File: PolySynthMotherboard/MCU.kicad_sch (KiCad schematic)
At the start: 46 parts, among them J201 SWD Header, J202 USB_C, J203 MIDI_In, J204 MIDI_Thru, J207 MIDI_Out, J401 Micro_SD_Card_Det2, SW201 RST, SW202 BOOT, U201 STM32F411RETx, U202 74HC595, U203 74HC595, U204 6N138, U205 74HC04, Y201 16MHz, Y202 32.768kHZ

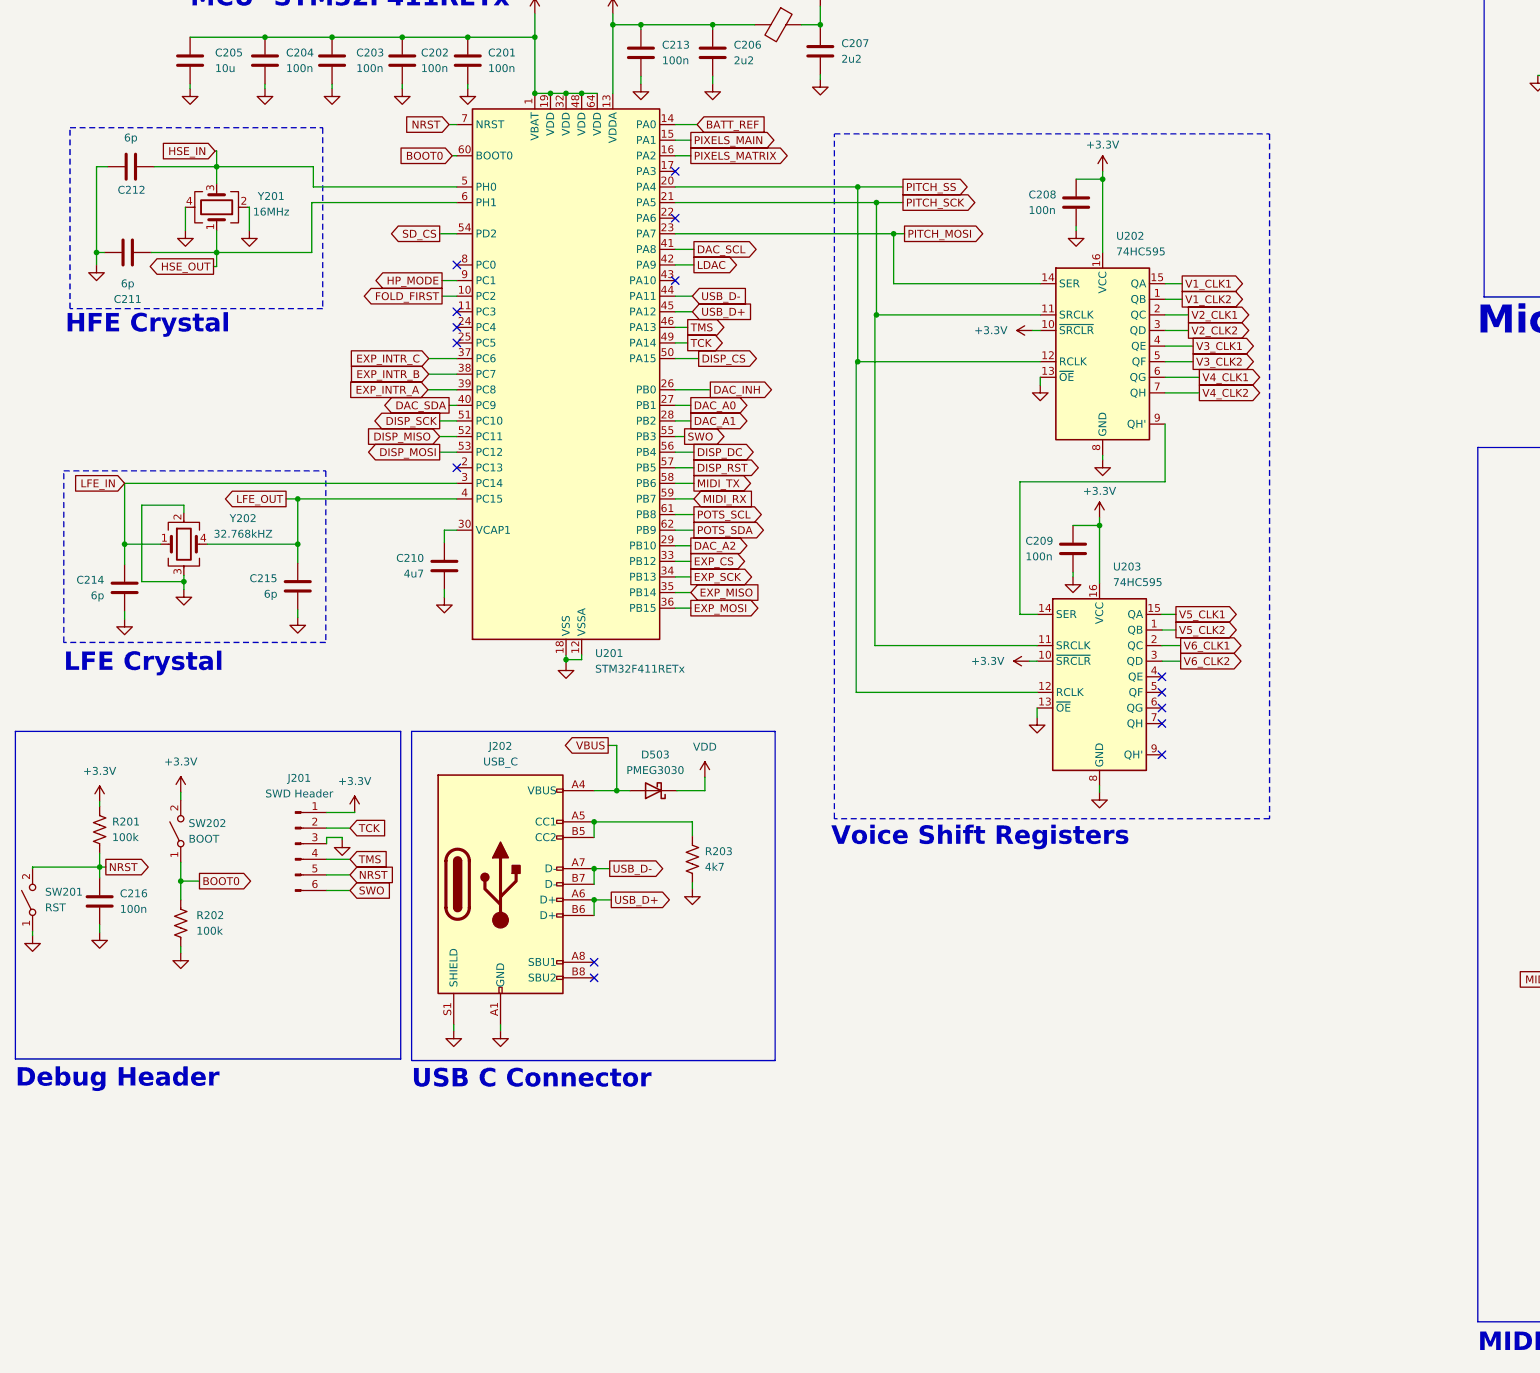
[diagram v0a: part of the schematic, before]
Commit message: added terminations
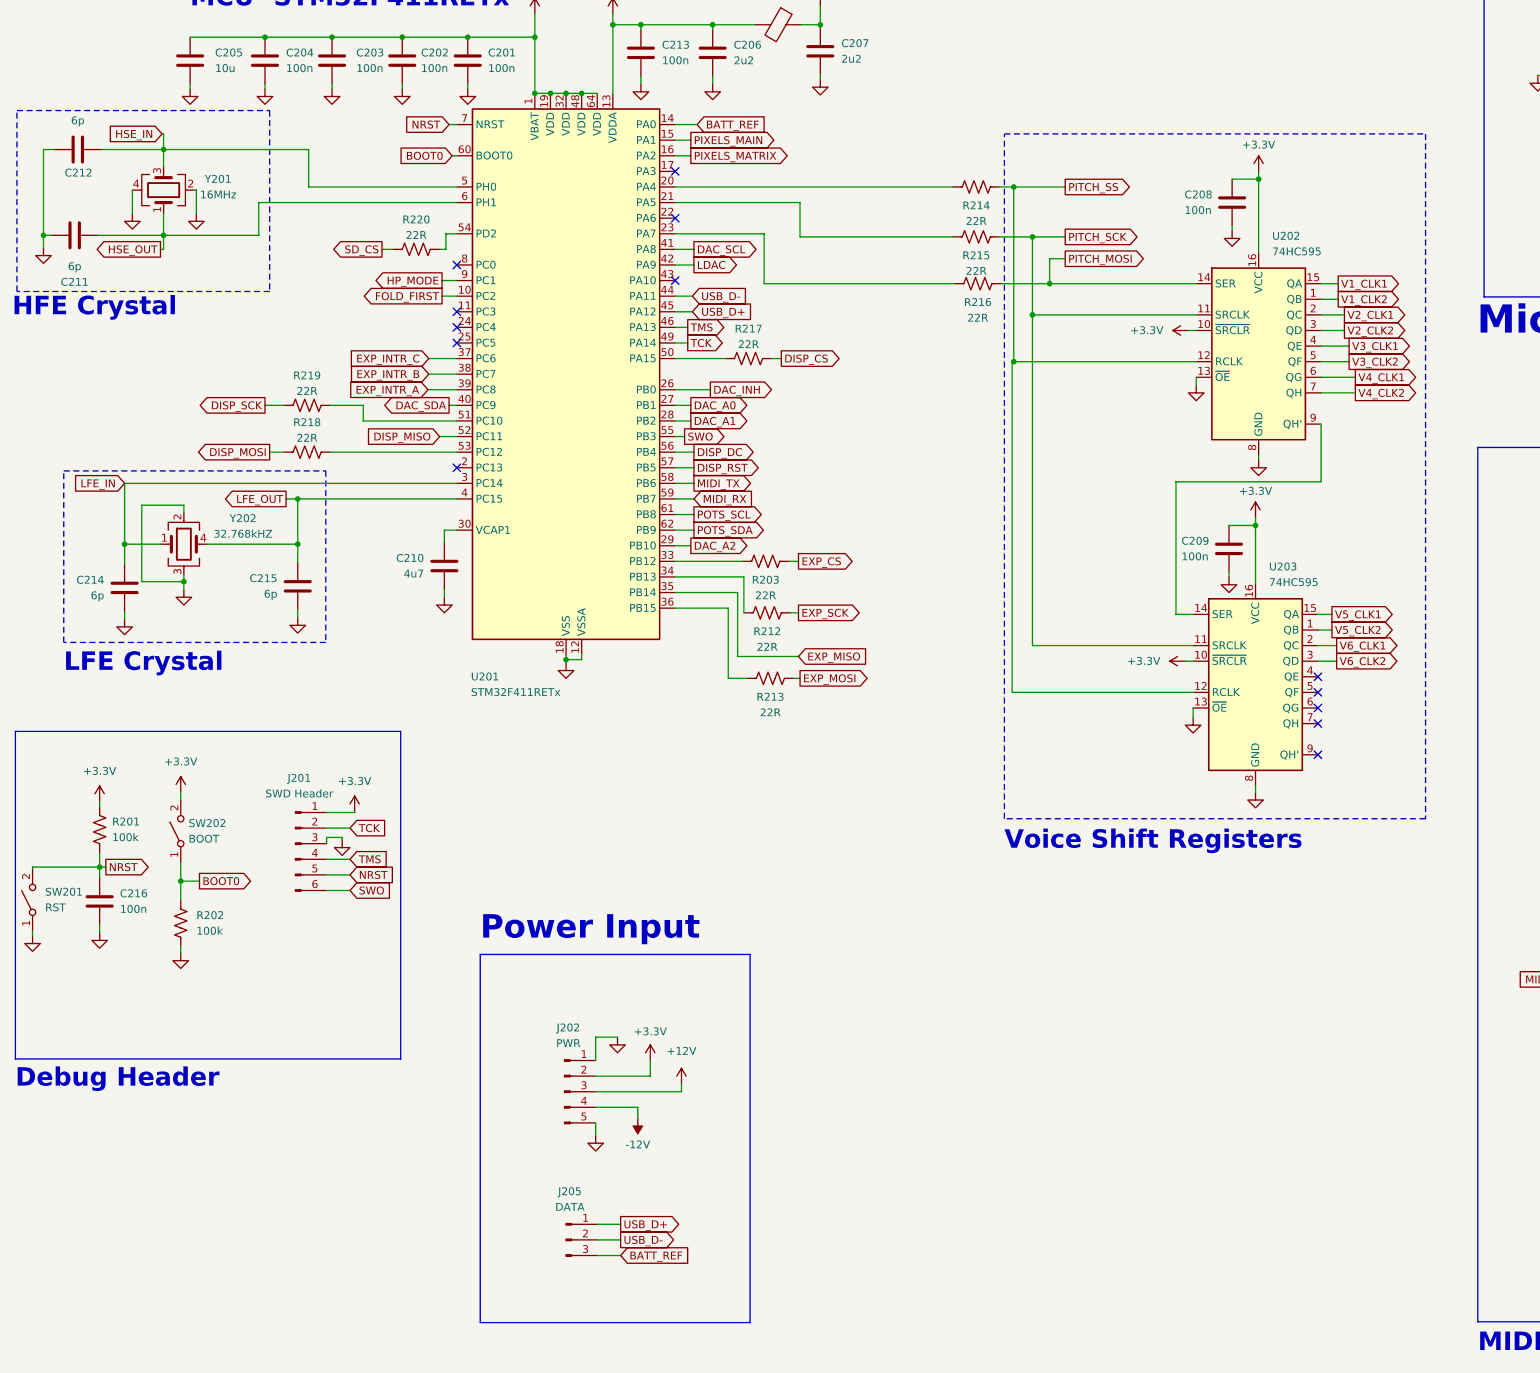
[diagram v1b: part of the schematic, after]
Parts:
- removed D503: PMEG3030, Diode_SMD:D_SOD-123, symbol Device:D_Schottky
- removed J202: USB_C, Connector_USB:USB_C_Receptacle_JAE_DX07S016JA1R1500, symbol Connector:USB_C_Receptacle_USB2.0
- added J202: PWR, Connector_PinHeader_2.54mm:PinHeader_1x05_P2.54mm_Vertical, symbol Connector:Conn_01x05_Pin
- added J205: DATA, Connector_PinHeader_2.54mm:PinHeader_1x03_P2.54mm_Vertical, symbol Connector:Conn_01x03_Pin
- added R212, R213, R214, R215, R216, R217, R218, R219, R220: 22R, Resistor_SMD:R_0805_2012Metric, symbol Device:R_US
- R203: value 4k7 -> 22R
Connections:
- net +3.3V: now also J202.2 (Pin_2)
- net BATT_REF: now also J205.3 (Pin_3)
- net DISP_CS: now also R217.2; no longer U201.50 (PA15)
- net DISP_MOSI: now also R218.1; no longer U201.53 (PC12)
- net DISP_SCK: now also R219.1; no longer U201.51 (PC10)
- net EXP_CS: now also R203.2; no longer U201.33 (PB12)
- net EXP_MOSI: now also R213.2; no longer U201.36 (PB15)
- net EXP_SCK: now also R212.2; no longer U201.34 (PB13)
- net GND: now also J202.1 (Pin_1), J202.5 (Pin_5); no longer R203.2
- net PITCH_MOSI: now also R216.2; no longer U201.23 (PA7)
- net PITCH_SCK: now also R215.2; no longer U201.21 (PA5)
- net PITCH_SS: now also R214.2; no longer U201.20 (PA4)
- net SD_CS: now also R220.1; no longer U201.54 (PD2)
- net USB_D+: now also J205.1 (Pin_1)
- net USB_D-: now also J205.2 (Pin_2)
- net at R203.1: now also U201.33 (PB12)
- new net: R212.1, U201.34 (PB13)
- new net: R216.1, U201.23 (PA7)
- new net: R214.1, U201.20 (PA4)
- new net: R213.1, U201.36 (PB15)
- new net: R215.1, U201.21 (PA5)
- new net: R217.1, U201.50 (PA15)
- new net: R219.2, U201.51 (PC10)
- new net: R218.2, U201.53 (PC12)
- new net: R220.2, U201.54 (PD2)
- new net +12V: J202.3 (Pin_3)
- new net -12V: J202.4 (Pin_4)
- no-connect marks 23 -> 21
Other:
- note added: "Power Input"
- note removed: "USB C Connector"
- moved on the sheet: C208, C209, C211, C212, U202, U203, Y201

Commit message: board iteration
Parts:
- removed R404: 47k, Resistor_SMD:R_0805_2012Metric, symbol Device:R_US
- added R210, R221, R222, R223, R224, R225, R226, R227: 22R, Resistor_SMD:R_0805_2012Metric, symbol Device:R_US
- added R228, R229, R230: 47k, Resistor_SMD:R_0805_2012Metric, symbol Device:R_US
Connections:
- net +3.3V: now also R228.1, R229.1, R230.1
- net DISP_DC: now also R227.2; no longer U201.56 (PB4)
- net DISP_MISO: now also R225.2; no longer J401.7 (DAT0)
- net EXP_CS: now also R230.2
- net PITCH_SS: now also R229.2
- net PIXELS_MAIN: now also R226.2; no longer U201.15 (PA1)
- net PIXELS_MATRIX: now also R210.2; no longer U201.16 (PA2)
- net SD_CS: now also R228.2
- net DAC_A0: no longer names the net of U201.27 (PB1)
- net DAC_A0: now also R222.1
- net DAC_A1: no longer names the net of U201.28 (PB2)
- net DAC_A1: now also R223.1
- net DAC_A2: no longer names the net of U201.29 (PB10)
- net DAC_A2: now also R224.1
- net DAC_INH: no longer names the net of U201.26 (PB0)
- net DAC_INH: now also R221.1
- new net: R226.1, U201.15 (PA1)
- new net: R210.1, U201.16 (PA2)
- new net: R227.1, U201.56 (PB4)
- new net: J401.7 (DAT0), R225.1
- new net MUX_A0: R222.2
- new net MUX_A1: R223.2
- new net MUX_A2: R224.2
- new net MUX_INH: R221.2
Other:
- note added: "CV multiplexer control"
- note added: "Neopixels"
- note added: "Note: not sure if these terminations are necessary but the traces are long so they're here just in case"
- note added: "Port Expander Bus"
- moved on the sheet: C208, C209, C216, C217, D201, J201, J202, J203, J204, J205, J207, J401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
